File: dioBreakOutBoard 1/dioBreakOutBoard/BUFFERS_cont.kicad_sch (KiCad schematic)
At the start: 24 parts, among them U1 SN74LVC8T245QPWRQ1, U2 SN74LVC8T245QPWRQ1, U3 SN74LVC8T245QPWRQ1, U4 SN74LVC8T245QPWRQ1

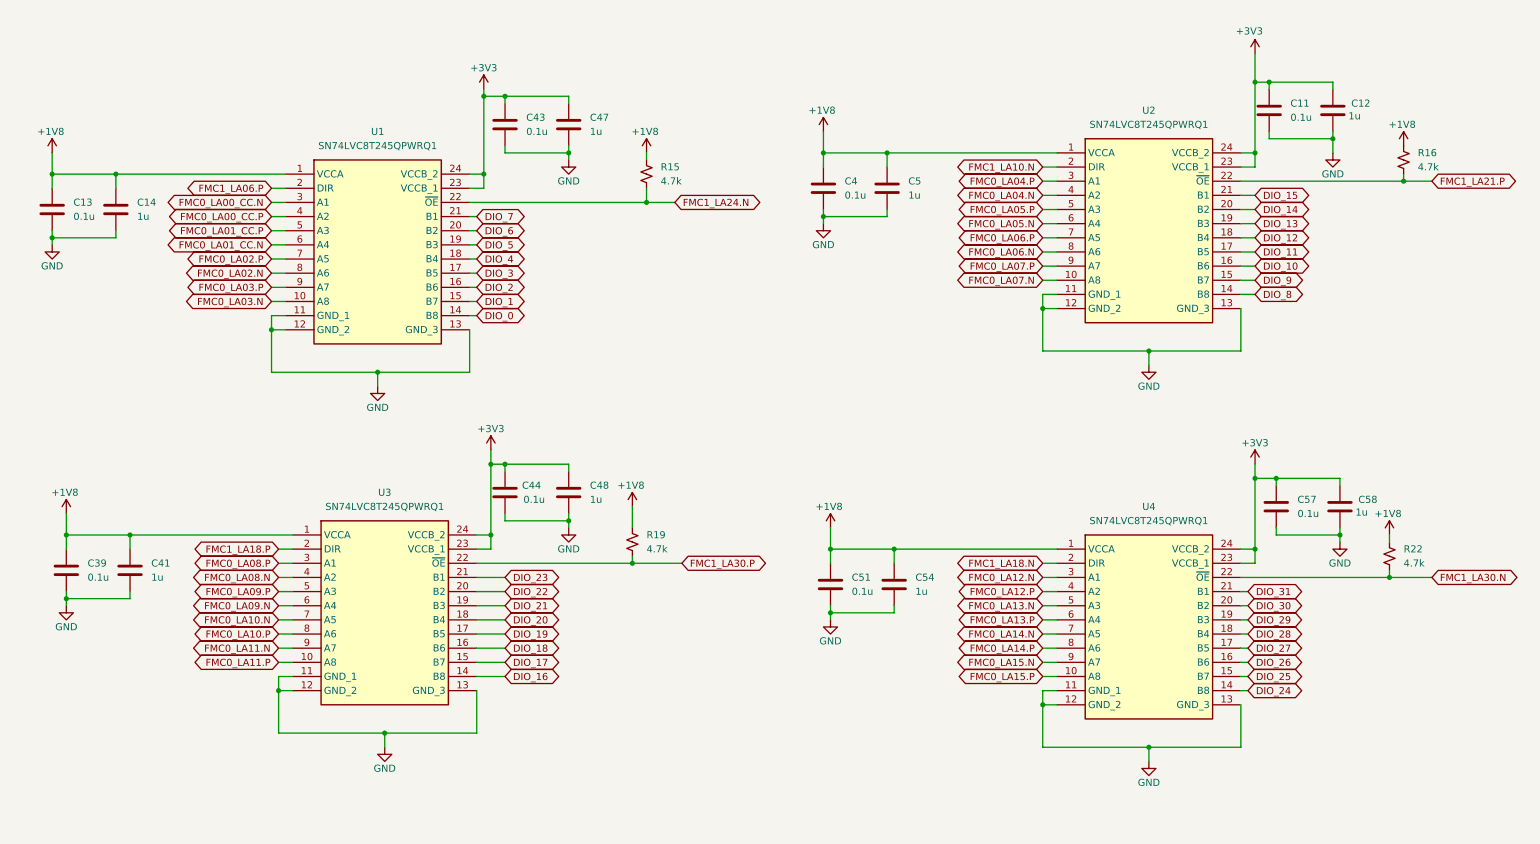
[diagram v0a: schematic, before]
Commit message: C:\Users\khernandez\KiCad\KiCad-Projects# Please enter the commit message for your changes. Lines starting
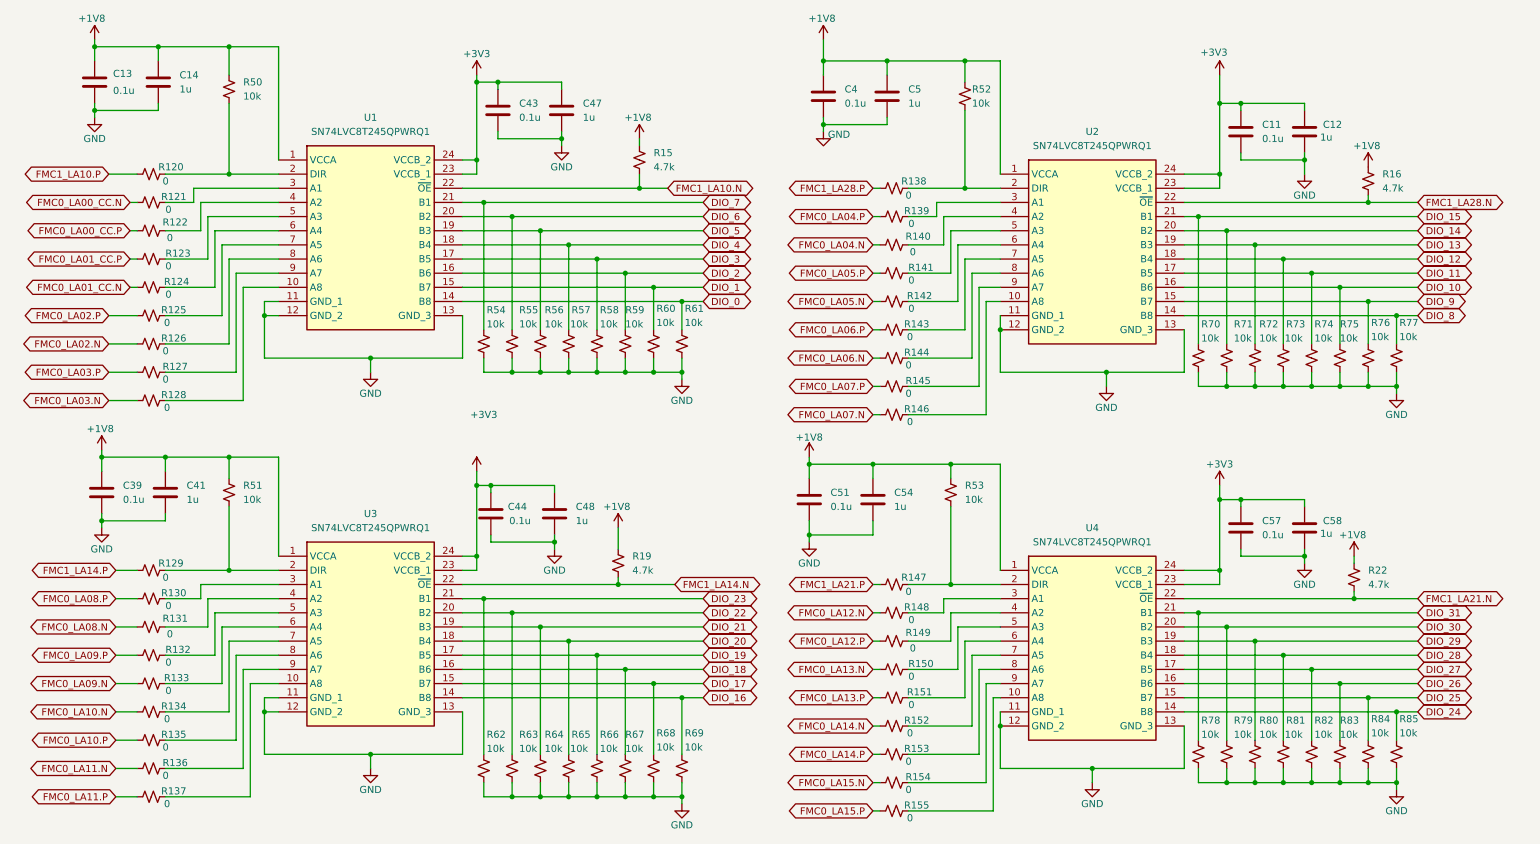
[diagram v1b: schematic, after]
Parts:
- added R120, R121, R122, R123, R124, R125, R126, R127, R128, R129, R130, R131, R132, R133, R134, R135, R136, R137, R138, R139, R140, R141, R142, R143, R144, R145, R146, R147, R148, R149, R150, R151, R152, R153, R154, R155: 0, Resistor_SMD:R_0603_1608Metric, symbol Device:R_Small_US
- added R50, R51, R52, R53, R54, R55, R56, R57, R58, R59, R60, R61, R62, R63, R64, R65, R66, R67, R68, R69, R70, R71, R72, R73, R74, R75, R76, R77, R78, R79, R80, R81, R82, R83, R84, R85: 10k, Resistor_SMD:R_0603_1608Metric, symbol Device:R_Small_US
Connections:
- net FMC1_LA24.N is gone; now on net FMC1_LA10.N: R15.1, U1.22 (~{OE})
- net +1V8: now also R50.2, R51.2, R52.2, R53.2
- net DIO_0: now also R61.2
- net DIO_1: now also R60.2
- net DIO_10: now also R75.2
- net DIO_11: now also R74.2
- net DIO_12: now also R73.2
- net DIO_13: now also R72.2
- net DIO_14: now also R71.2
- net DIO_15: now also R70.2
- net DIO_16: now also R69.2
- net DIO_17: now also R68.2
- net DIO_18: now also R67.2
- net DIO_19: now also R66.2
- net DIO_2: now also R59.2
- net DIO_20: now also R65.2
- net DIO_21: now also R64.2
- net DIO_22: now also R63.2
- net DIO_23: now also R62.2
- net DIO_24: now also R85.2
- net DIO_25: now also R84.2
- net DIO_26: now also R83.2
- net DIO_27: now also R82.2
- net DIO_28: now also R81.2
- net DIO_29: now also R80.2
- net DIO_3: now also R58.2
- net DIO_30: now also R79.2
- net DIO_31: now also R78.2
- net DIO_4: now also R57.2
- net DIO_5: now also R56.2
- net DIO_6: now also R55.2
- net DIO_7: now also R54.2
- net DIO_8: now also R77.2
- net DIO_9: now also R76.2
- net FMC0_LA00_CC.N: now also R121.1; no longer U1.3 (A1)
- net FMC0_LA00_CC.P: now also R122.1; no longer U1.4 (A2)
- net FMC0_LA01_CC.N: now also R124.1; no longer U1.6 (A4)
- net FMC0_LA01_CC.P: now also R123.1; no longer U1.5 (A3)
- net FMC0_LA02.N: now also R126.1; no longer U1.8 (A6)
- net FMC0_LA02.P: now also R125.1; no longer U1.7 (A5)
- net FMC0_LA03.N: now also R128.1; no longer U1.10 (A8)
- net FMC0_LA03.P: now also R127.1; no longer U1.9 (A7)
- net FMC0_LA04.N: now also R140.1; no longer U2.4 (A2)
- net FMC0_LA04.P: now also R139.1; no longer U2.3 (A1)
- net FMC0_LA05.N: now also R142.1; no longer U2.6 (A4)
- net FMC0_LA05.P: now also R141.1; no longer U2.5 (A3)
- net FMC0_LA06.N: now also R144.1; no longer U2.8 (A6)
- net FMC0_LA06.P: now also R143.1; no longer U2.7 (A5)
- net FMC0_LA07.N: now also R146.1; no longer U2.10 (A8)
- net FMC0_LA07.P: now also R145.1; no longer U2.9 (A7)
- net FMC0_LA08.N: now also R131.1; no longer U3.4 (A2)
- net FMC0_LA08.P: now also R130.1; no longer U3.3 (A1)
- net FMC0_LA09.N: now also R133.1; no longer U3.6 (A4)
- net FMC0_LA09.P: now also R132.1; no longer U3.5 (A3)
- net FMC0_LA10.N: now also R134.1; no longer U3.7 (A5)
- net FMC0_LA10.P: now also R135.1; no longer U3.8 (A6)
- net FMC0_LA11.N: now also R136.1; no longer U3.9 (A7)
- net FMC0_LA11.P: now also R137.1; no longer U3.10 (A8)
- net FMC0_LA12.N: now also R148.1; no longer U4.3 (A1)
- net FMC0_LA12.P: now also R149.1; no longer U4.4 (A2)
- net FMC0_LA13.N: now also R150.1; no longer U4.5 (A3)
- net FMC0_LA13.P: now also R151.1; no longer U4.6 (A4)
- net FMC0_LA14.N: now also R152.1; no longer U4.7 (A5)
- net FMC0_LA14.P: now also R153.1; no longer U4.8 (A6)
- net FMC0_LA15.N: now also R154.1; no longer U4.9 (A7)
- net FMC0_LA15.P: now also R155.1; no longer U4.10 (A8)
- net FMC1_LA10.N: no longer U2.2 (DIR)
- net FMC1_LA21.P: now also R147.1; no longer R16.1, U2.22 (~{OE})
- net GND: now also R54.1, R55.1, R56.1, R57.1, R58.1, R59.1, R60.1, R61.1, R62.1, R63.1, R64.1, R65.1, R66.1, R67.1, R68.1, R69.1, R70.1, R71.1, R72.1, R73.1, R74.1, R75.1, R76.1, R77.1, R78.1, R79.1, R80.1, R81.1, R82.1, R83.1, R84.1, R85.1
- net FMC1_LA06.P: no longer names the net of U1.2 (DIR)
- net FMC1_LA06.P: now also R120.2, R50.1
- net FMC1_LA18.N: no longer names the net of U4.2 (DIR)
- net FMC1_LA18.N: now also R147.2, R53.1
- net FMC1_LA18.P: no longer names the net of U3.2 (DIR)
- net FMC1_LA18.P: now also R129.2, R51.1
- net FMC1_LA30.N renamed FMC1_LA21.N
- net FMC1_LA30.P renamed FMC1_LA14.N
- new net: R134.2, U3.7 (A5)
- new net: R135.2, U3.8 (A6)
- new net: R151.2, U4.6 (A4)
- new net: R142.2, U2.6 (A4)
- new net: R133.2, U3.6 (A4)
- new net: R153.2, U4.8 (A6)
- new net: R155.2, U4.10 (A8)
- new net: R148.2, U4.3 (A1)
- new net: R123.2, U1.5 (A3)
- new net: R141.2, U2.5 (A3)
- new net: R136.2, U3.9 (A7)
- new net: R143.2, U2.7 (A5)
- new net: R146.2, U2.10 (A8)
- new net: R138.2, R52.1, U2.2 (DIR)
- new net: R139.2, U2.3 (A1)
- new net: R140.2, U2.4 (A2)
- new net: R144.2, U2.8 (A6)
- new net: R145.2, U2.9 (A7)
- new net: R130.2, U3.3 (A1)
- new net: R150.2, U4.5 (A3)
- new net: R121.2, U1.3 (A1)
- new net: R128.2, U1.10 (A8)
- new net: R122.2, U1.4 (A2)
- new net: R124.2, U1.6 (A4)
- new net: R125.2, U1.7 (A5)
- new net: R126.2, U1.8 (A6)
- new net: R127.2, U1.9 (A7)
- new net: R131.2, U3.4 (A2)
- new net: R152.2, U4.7 (A5)
- new net: R154.2, U4.9 (A7)
- new net: R149.2, U4.4 (A2)
- new net: R132.2, U3.5 (A3)
- new net: R137.2, U3.10 (A8)
- new net FMC1_LA10.P: R120.1
- new net FMC1_LA14.P: R129.1
- new net FMC1_LA28.N: R16.1, U2.22 (~{OE})
- new net FMC1_LA28.P: R138.1
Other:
- moved on the sheet: C11, C12, C13, C14, C39, C4, C41, C43, C44, C47, C48, C5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

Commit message: added 2 bit buffers, which replace the previous 8 bit buffers
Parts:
- removed C11, C13, C39, C4, C43, C44, C51, C57: 0.1u, Capacitor_SMD:C_0603_1608Metric, symbol Device:C
- removed C12, C14, C41, C47, C48, C5, C54, C58: 1u, Capacitor_SMD:C_0805_2012Metric_Pad1.18x1.45mm_HandSolder, symbol Device:C
- removed R120, R121, R122, R123, R124, R125, R126, R127, R128, R129, R130, R131: 0, Resistor_SMD:R_0603_1608Metric, symbol Device:R_Small_US
- removed R15, R16, R19, R22: 4.7k, Resistor_SMD:R_0603_1608Metric, symbol Device:R_Small_US
- removed R50, R51, R52, R53, R54, R55, R56, R57, R58, R59, R60, R61, R62, R63, R64, R65, R66, R67, R68, R69, R70, R71, R72, R73, R74, R75, R76, R77, R78, R79, R80, R81, R82, R83, R84, R85: 10k, Resistor_SMD:R_0603_1608Metric, symbol Device:R_Small_US
- removed U1, U3, U4: SN74LVC8T245QPWRQ1, SOP65P640X120-24N, symbol SN74LVC8T245QPWRQ1:SN74LVC8T245QPWRQ1
- removed U2: SN74LVC8T245QPWRQ1, LevelShifters:SOP65P640X120-24N, symbol SN74LVC8T245QPWRQ1:SN74LVC8T245QPWRQ1
- added C100, C107, C108, C109, C110, C111, C112, C119, C120, C121, C122, C127, C128, C129, C130, C71, C72, C73, C74, C75, C76, C83, C84, C85, C86, C87, C88, C95, C96, C97, C98, C99: 0.1u, Capacitor_SMD:C_0603_1608Metric, symbol Device:C
- added C101, C102, C103, C104, C105, C106, C113, C114, C115, C116, C117, C118, C123, C124, C125, C126, C131, C132, C133, C134, C77, C78, C79, C80, C81, C82, C89, C90, C91, C92, C93, C94: 1u, Capacitor_SMD:C_0805_2012Metric_Pad1.18x1.45mm_HandSolder, symbol Device:C
- added IC18, IC19, IC20, IC21, IC22, IC23, IC24, IC25, IC26, IC27, IC28, IC29, IC30, IC31, IC32, IC33: SN74LVC2T45QDCURQ1, LevelShifters:SN74LVC2T45-Q1, symbol SN74LVC2T45QDCURQ1:SN74LVC2T45QDCURQ1
- added R156, R157, R158, R159, R160, R161, R162, R163, R164, R165, R166, R167, R180, R181, R182, R183, R184, R185, R186, R187, R188, R189, R190, R191, R192, R194, R198, R201, R202, R203, R204, R205, R206, R207, R208, R209, R210, R211, R212, R213, R214, R215, R228, R229, R230, R231, R232, R233, R234, R235, R236, R237, R242, R243, R244, R245, R246, R247, R248, R249, R250, R251: 0, Resistor_SMD:R_0603_1608Metric, symbol Device:R_Small_US
- added R168, R169, R170, R171, R172, R173, R174, R175, R176, R177, R178, R179, R193, R195, R196, R197, R199, R200, R216, R217, R218, R219, R220, R221, R222, R223, R224, R225, R226, R227, R238, R239, R240, R241, R252, R253, R254, R255, R256, R257, R258, R259: 10k, Resistor_SMD:R_0603_1608Metric, symbol Device:R_Small_US
- R142, R143, R146, R148, R149, R153: value 0 -> 10k
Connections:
- net FMC1_LA28.P is gone; now on net FMC0_LA00_CC.N: R138.1
- net +1V8: now also R142.2, R143.2, R146.2, R148.2, R149.2, R153.2, C100.2, C101.2, C102.2, C103.2, C104.2, C105.2, C106.2, C119.2, C120.2, C121.2, C122.2, C123.2, C124.2, C125.2, C126.2, C71.2, C72.2, C73.2, C74.2, C75.2, C76.2, C77.2, C78.2, C79.2, C80.2, C81.2, C82.2, C95.2, C96.2, C97.2, C98.2, C99.2, IC18.1 (VCCA), IC19.1 (VCCA), IC20.1 (VCCA), IC21.1 (VCCA), IC22.1 (VCCA), IC23.1 (VCCA), IC24.1 (VCCA), IC25.1 (VCCA), IC26.1 (VCCA), IC27.1 (VCCA), IC28.1 (VCCA), IC29.1 (VCCA), IC30.1 (VCCA), IC31.1 (VCCA), IC32.1 (VCCA), IC33.1 (VCCA), R193.2, R195.2, R196.2, R197.2, R199.2, R200.2, R238.2, R239.2, R240.2, R241.2
- net +3V3: now also C107.2, C108.2, C109.2, C110.2, C111.2, C112.2, C113.2, C114.2, C115.2, C116.2, C117.2, C118.2, C127.2, C128.2, C129.2, C130.2, C131.2, C132.2, C133.2, C134.2, C83.2, C84.2, C85.2, C86.2, C87.2, C88.2, C89.2, C90.2, C91.2, C92.2, C93.2, C94.2, IC18.8 (VCCB), IC19.8 (VCCB), IC20.8 (VCCB), IC21.8 (VCCB), IC22.8 (VCCB), IC23.8 (VCCB), IC24.8 (VCCB), IC25.8 (VCCB), IC26.8 (VCCB), IC27.8 (VCCB), IC28.8 (VCCB), IC29.8 (VCCB), IC30.8 (VCCB), IC31.8 (VCCB), IC32.8 (VCCB), IC33.8 (VCCB)
- net DIO_0: now also R163.2, R175.2
- net DIO_1: now also R157.2, R169.2
- net DIO_10: now also R215.2, R227.2
- net DIO_11: now also R209.2, R221.2
- net DIO_12: now also R214.2, R226.2
- net DIO_13: now also R208.2, R220.2
- net DIO_14: now also R213.2, R225.2
- net DIO_15: now also R207.2, R219.2
- net DIO_16: now also R211.2, R222.2
- net DIO_17: now also R205.2, R216.2
- net DIO_18: now also R210.2, R223.2
- net DIO_19: now also R204.2, R217.2
- net DIO_2: now also R166.2, R174.2
- net DIO_20: now also R156.2, R176.2
- net DIO_21: now also R164.2, R170.2
- net DIO_22: now also R167.2, R178.2
- net DIO_23: now also R161.2, R171.2
- net DIO_24: now also R251.2, R259.2
- net DIO_25: now also R247.2, R255.2
- net DIO_26: now also R250.2, R258.2
- net DIO_27: now also R246.2, R254.2
- net DIO_28: now also R249.2, R257.2
- net DIO_29: now also R245.2, R253.2
- net DIO_3: now also R159.2, R168.2
- net DIO_30: now also R248.2, R256.2
- net DIO_31: now also R244.2, R252.2
- net DIO_4: now also R162.2, R179.2
- net DIO_5: now also R158.2, R173.2
- net DIO_6: now also R165.2, R177.2
- net DIO_7: now also R160.2, R172.2
- net DIO_8: now also R212.2, R224.2
- net DIO_9: now also R206.2, R218.2
- net FMC0_LA00_CC.P: now also R145.1
- net FMC0_LA01_CC.N: now also R154.1
- net FMC0_LA01_CC.P: now also R147.1
- net FMC0_LA02.N: now also R155.1
- net FMC0_LA02.P: now also R144.1
- net FMC0_LA03.N: now also R152.1
- net FMC0_LA03.P: now also R141.1
- net FMC0_LA04.N: now also R201.1; no longer R140.1
- net FMC0_LA04.P: now also R188.1; no longer R139.1
- net FMC0_LA05.N: now also R189.1; no longer R142.1
- net FMC0_LA05.P: now also R202.1; no longer R141.1
- net FMC0_LA06.N: now also R203.1; no longer R144.1
- net FMC0_LA06.P: now also R190.1; no longer R143.1
- net FMC0_LA07.N: now also R198.1; no longer R146.1
- net FMC0_LA07.P: now also R191.1; no longer R145.1
- net FMC0_LA08.N: now also R151.1
- net FMC0_LA08.P: now also R140.1
- net FMC0_LA09.N: now also R150.1; no longer R133.1
- net FMC0_LA09.P: now also R139.1; no longer R132.1
- net FMC0_LA10.N: now also R187.1; no longer R134.1
- net FMC0_LA10.P: now also R194.1; no longer R135.1
- net FMC0_LA11.N: now also R186.1; no longer R136.1
- net FMC0_LA11.P: now also R192.1; no longer R137.1
- net FMC0_LA12.N: now also R234.1; no longer R148.1
- net FMC0_LA12.P: now also R242.1; no longer R149.1
- net FMC0_LA13.N: now also R232.1; no longer R150.1
- net FMC0_LA13.P: now also R236.1; no longer R151.1
- net FMC0_LA14.N: now also R233.1; no longer R152.1
- net FMC0_LA14.P: now also R237.1; no longer R153.1
- net FMC0_LA15.N: now also R235.1; no longer R154.1
- net FMC0_LA15.P: now also R243.1; no longer R155.1
- net FMC1_LA10.N: now also R137.1
- net FMC1_LA10.P: now also R133.2
- net FMC1_LA14.N: now also R134.1
- net FMC1_LA14.P: now also R136.2
- net FMC1_LA21.P: no longer R147.1
- net GND: now also C100.1, C101.1, C102.1, C103.1, C104.1, C105.1, C106.1, C107.1, C108.1, C109.1, C110.1, C111.1, C112.1, C113.1, C114.1, C115.1, C116.1, C117.1, C118.1, C119.1, C120.1, C121.1, C122.1, C123.1, C124.1, C125.1, C126.1, C127.1, C128.1, C129.1, C130.1, C131.1, C132.1, C133.1, C134.1, C71.1, C72.1, C73.1, C74.1, C75.1, C76.1, C77.1, C78.1, C79.1, C80.1, C81.1, C82.1, C83.1, C84.1, C85.1, C86.1, C87.1, C88.1, C89.1, C90.1, C91.1, C92.1, C93.1, C94.1, C95.1, C96.1, C97.1, C98.1, C99.1, IC18.4 (GND), IC19.4 (GND), IC20.4 (GND), IC21.4 (GND), IC22.4 (GND), IC23.4 (GND), IC24.4 (GND), IC25.4 (GND), IC26.4 (GND), IC27.4 (GND), IC28.4 (GND), IC29.4 (GND), IC30.4 (GND), IC31.4 (GND), IC32.4 (GND), IC33.4 (GND), R168.1, R169.1, R170.1, R171.1, R172.1, R173.1, R174.1, R175.1, R176.1, R177.1, R178.1, R179.1, R216.1, R217.1, R218.1, R219.1, R220.1, R221.1, R222.1, R223.1, R224.1, R225.1, R226.1, R227.1, R252.1, R253.1, R254.1, R255.1, R256.1, R257.1, R258.1, R259.1
- net at R134.2: now also R142.1, IC20.5 (DIR)
- net at R135.2: now also R153.1, IC23.5 (DIR)
- net at R151.2: now also IC23.3 (A2)
- net at R147.2: now also IC21.2 (A1)
- net at R155.2: now also IC22.3 (A2)
- net at R141.2: now also IC20.2 (A1)
- net at R138.2: now also IC19.2 (A1)
- net at R139.2: now also IC18.2 (A1)
- net at R140.2: now also IC23.2 (A1)
- net at R144.2: now also IC22.2 (A1)
- net at R145.2: now also IC19.3 (A2)
- net at R150.2: now also IC18.3 (A2)
- net at R152.2: now also IC20.3 (A2)
- net at R154.2: now also IC21.3 (A2)
- net at R132.2: now also R148.1, IC18.5 (DIR)
- net at R137.2: now also R146.1, IC21.5 (DIR)
- new net: IC31.7 (B1), R245.1
- new net: IC31.2 (A1), R232.2
- new net: IC31.3 (A2), R236.2
- new net: IC31.5 (DIR), R229.2, R239.1
- new net: IC31.6 (B2), R249.1
- new net: IC33.5 (DIR), R231.2, R241.1
- new net: IC28.6 (B2), R214.1
- new net: IC24.3 (A2), R194.2
- new net: IC19.5 (DIR), R133.1, R149.1
- new net: IC24.2 (A1), R187.2
- new net: IC24.5 (DIR), R180.1, R199.1
- new net: IC24.6 (B2), R210.1
- new net: IC24.7 (B1), R204.1
- new net: IC26.2 (A1), R191.2
- new net: IC26.3 (A2), R198.2
- new net: IC26.5 (DIR), R185.2
- new net: IC26.6 (B2), R212.1
- new net: IC26.7 (B1), R206.1
- new net: IC22.5 (DIR), R136.1, R143.1
- new net: IC29.7 (B1), R209.1
- new net: IC21.6 (B2), R162.1
- new net: IC32.2 (A1), R234.2
- new net: IC32.3 (A2), R242.2
- new net: IC32.5 (DIR), R228.2, R238.1
- new net: IC32.6 (B2), R248.1
- new net: IC32.7 (B1), R244.1
- new net: IC30.5 (DIR), R230.2, R240.1
- new net: IC27.5 (DIR), R182.2, R195.1
- new net: IC18.7 (B1), R164.1
- new net: IC28.3 (A2), R202.2
- new net: IC19.6 (B2), R165.1
- new net: IC28.2 (A1), R189.2
- new net: IC25.5 (DIR), R181.1, R200.1
- new net: IC19.7 (B1), R160.1
- new net: IC28.5 (DIR), R183.2, R196.1
- new net: IC28.7 (B1), R208.1
- new net: IC30.7 (B1), R246.1
- new net: IC27.6 (B2), R213.1
- new net: IC30.2 (A1), R233.2
- new net: IC30.3 (A2), R237.2
- new net: IC30.6 (B2), R250.1
- new net: IC23.6 (B2), R167.1
- new net: IC23.7 (B1), R161.1
- new net: IC22.6 (B2), R166.1
- new net: IC20.7 (B1), R157.1
- new net: IC29.5 (DIR), R184.2, R197.1
- new net: IC27.7 (B1), R207.1
- new net: IC22.7 (B1), R159.1
- new net: IC25.2 (A1), R186.2
- new net: IC29.2 (A1), R190.2
- new net: IC29.3 (A2), R203.2
- new net: IC29.6 (B2), R215.1
- new net: IC21.7 (B1), R158.1
- new net: IC20.6 (B2), R163.1
- new net: IC25.7 (B1), R205.1
- new net: IC33.2 (A1), R235.2
- new net: IC33.3 (A2), R243.2
- new net: IC33.6 (B2), R251.1
- new net: IC33.7 (B1), R247.1
- new net: IC18.6 (B2), R156.1
- new net: IC25.3 (A2), R192.2
- new net: IC27.2 (A1), R188.2
- new net: IC25.6 (B2), R211.1
- new net: IC27.3 (A2), R201.2
- new net FMC1_LA02.N: R184.1
- new net FMC1_LA02.P: R185.1
- new net FMC1_LA04.P: R183.1
- new net FMC1_LA07.N: R182.1
- new net FMC1_LA11.N: R135.1
- new net FMC1_LA11.P: R181.2
- new net FMC1_LA13.N: R231.1
- new net FMC1_LA13.P: R180.2
- new net FMC1_LA15.N: R230.1
- new net FMC1_LA15.P: R132.1
- new net FMC1_LA17_CC.P: R229.1
- new net FMC1_LA19.P: R228.1
